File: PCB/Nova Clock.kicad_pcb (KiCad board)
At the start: 2 copper layers, 90.4 x 61.5 mm, 11 parts, among them J1 Conn_01x08_Pin, SW1 SW_Push, SW2 SW_Push, SW3 SW_Push, SW4 SW_Push, U1 XIAO-ESP32-C3-SMD

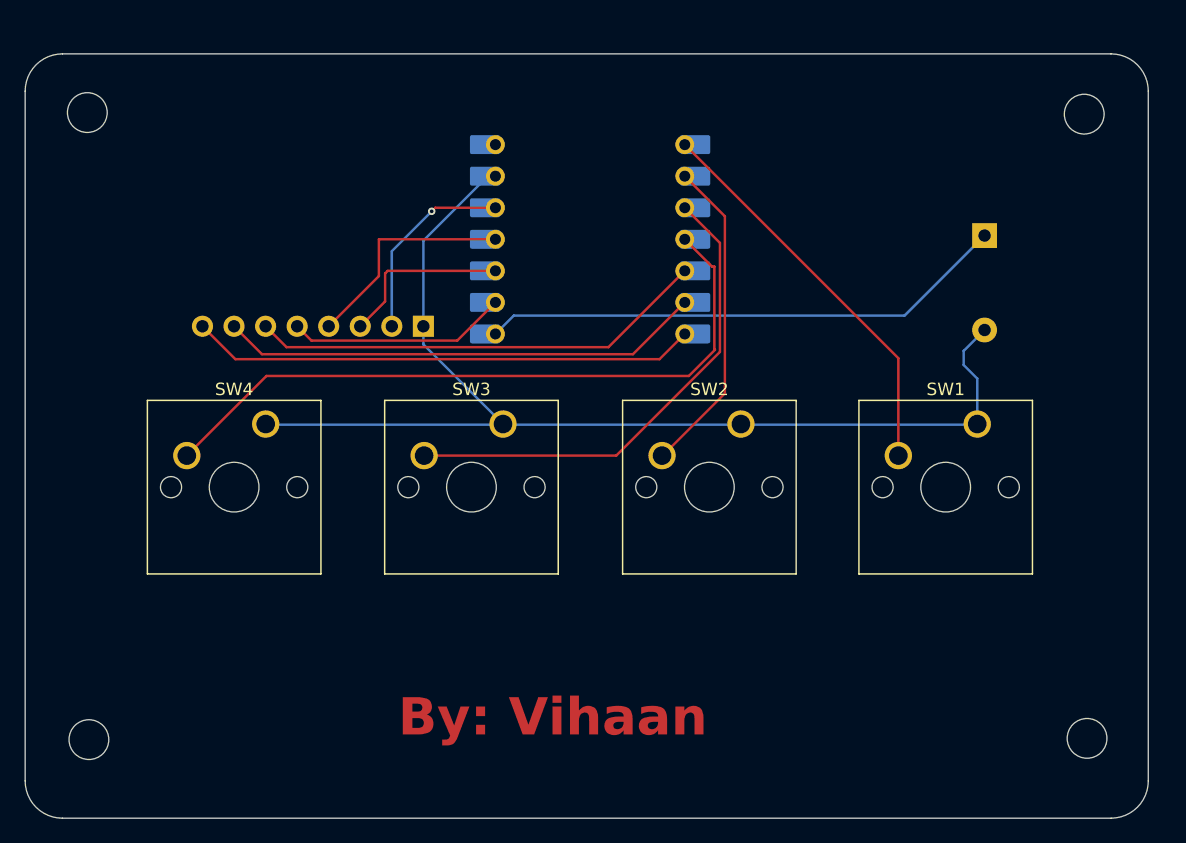
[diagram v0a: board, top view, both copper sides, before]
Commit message: Nova-Clock V2
In this commit, there is new PCB design, new case, and new images also added with a new are better firmware
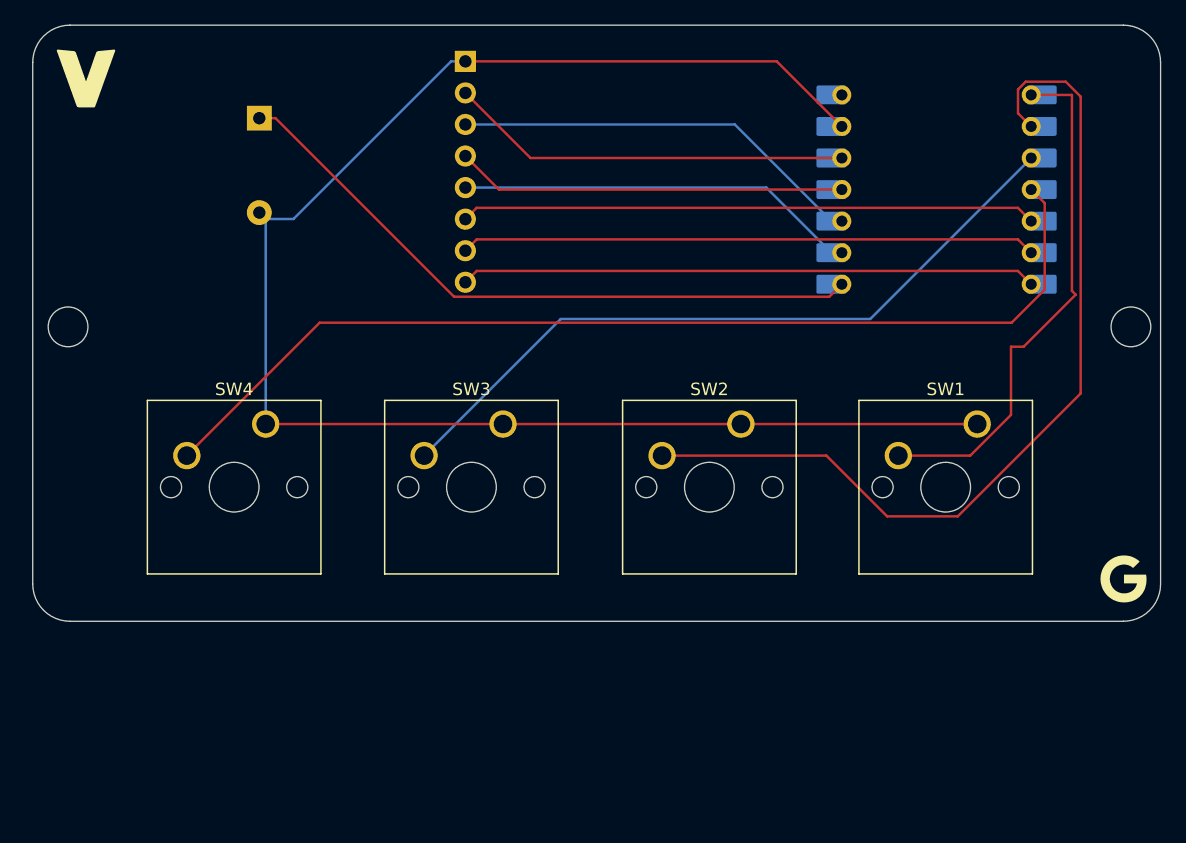
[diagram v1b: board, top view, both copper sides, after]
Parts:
- removed H1, H4: MountingHole, MountingHole:MountingHole_3.2mm_M3
- moved BZ1 59.1 mm to (112.4, 70.1)
- moved H3 33.3 mm to (182.6, 86.9)
- moved H2 33.3 mm to (97.1, 86.9)
- moved U1 28.2 mm to (167.0, 75.8)
- moved J1 21.6 mm to (129.0, 65.5), turned to 180 degrees
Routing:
- net Net-(U1-D1): track 26.0 -> 73.8 mm
- net GND: track 91.2 -> 129.1 mm, vias 1 -> 0
- net Net-(U1-D3): track 56.0 -> 83.9 mm
- net Net-(U1-D2): track 40.0 -> 59.6 mm
- net /SCL: track 14.0 -> 33.5 mm
- net +3.3V: track 15.5 -> 33.3 mm, vias 1 -> 0
- net /RST: track 17.7 -> 32.5 mm
- net /SDA: track 18.1 -> 32.3 mm
- net Net-(BZ1-+): track 42.7 -> 54.1 mm
- net /DC: track 37.0 -> 47.2 mm
- net Net-(U1-D0): track 33.1 -> 43.2 mm
- net /CS: track 38.9 -> 47.2 mm
- net /BL: track 40.8 -> 47.2 mm
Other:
- board size 90.4 x 61.5 mm -> 90.8 x 48 mm
- board text removed: "By: Vihaan"
